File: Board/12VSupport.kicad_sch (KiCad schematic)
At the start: 33 parts, among them J1 12V, J2 BATT, J3 BUCK_IN, J4 BUCK_OUT, J5 BOOST_IN, J6 BOOST_OUT, J8 HEATER, K1 SLA-05VDC-SL-C, K2 SLA-05VDC-SL-C, K3 SLA-05VDC-SL-C, K4 SLA-05VDC-SL-C, Q1 BSS138, Q2 BSS138, Q3 MMBF170, Q4 IRLR7843, U1 LM2596S-5, U4 ACS712xLCTR-20A

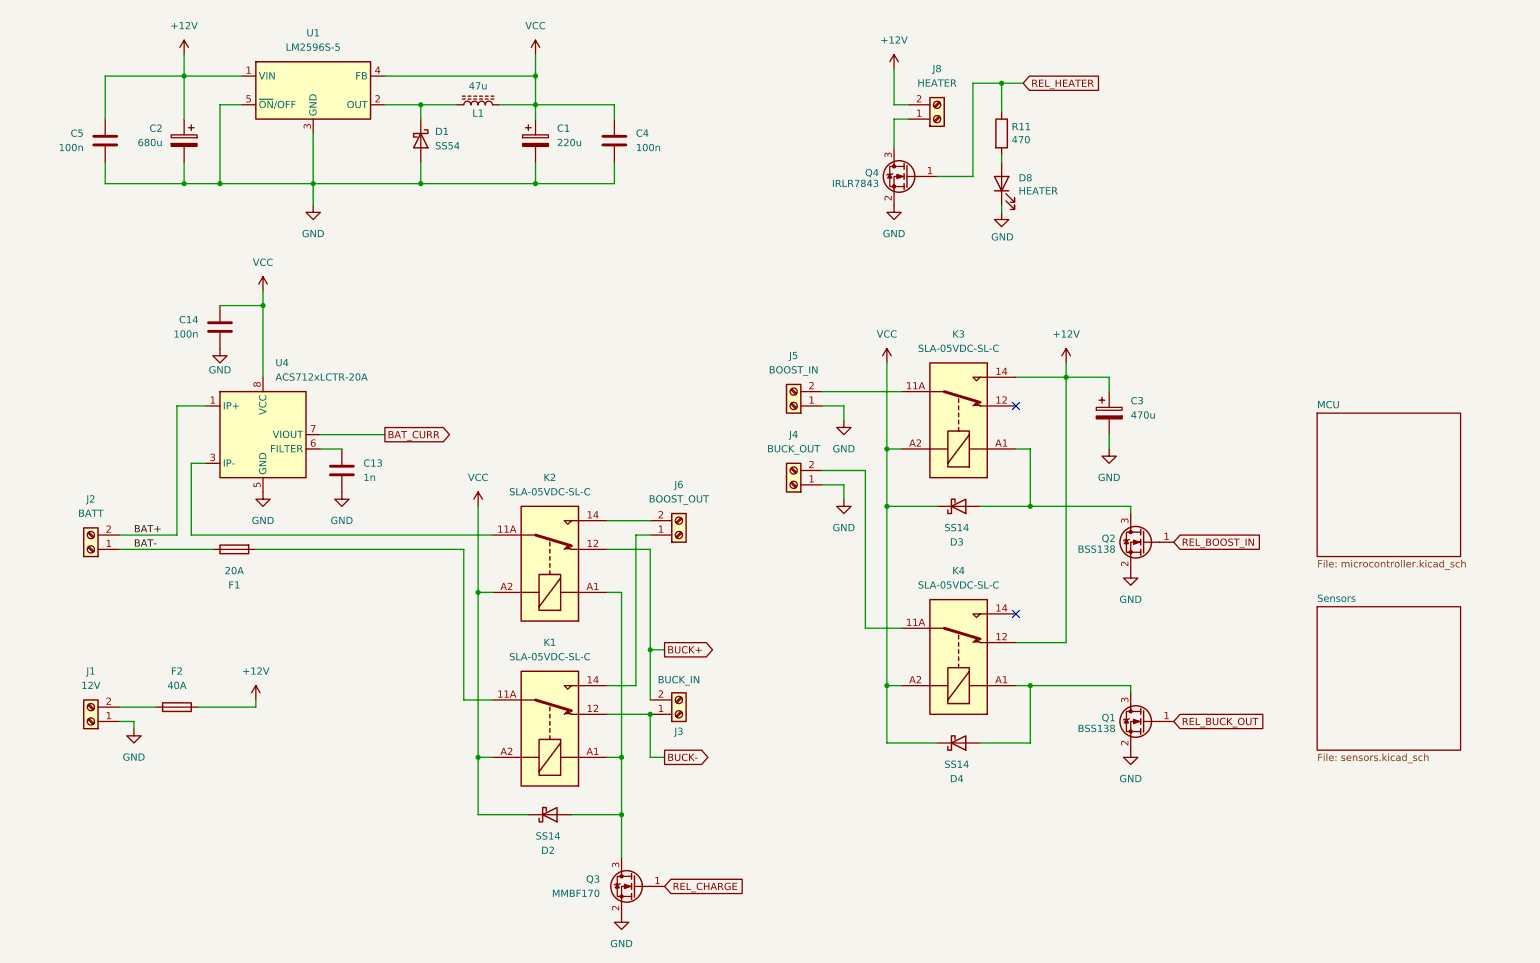
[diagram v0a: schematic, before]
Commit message: WIP
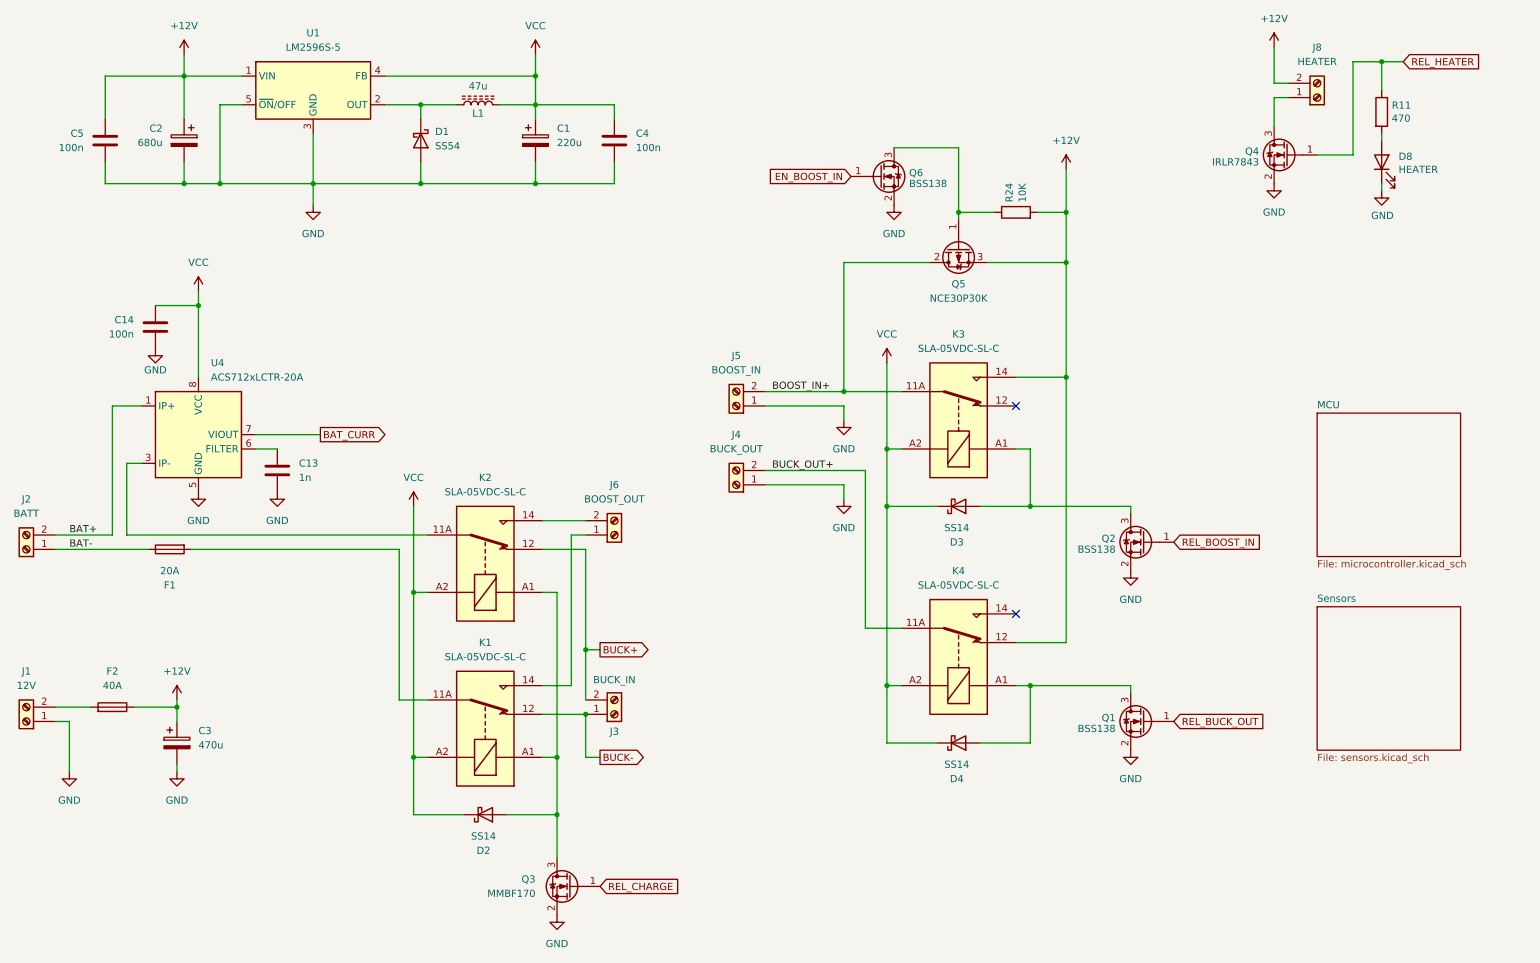
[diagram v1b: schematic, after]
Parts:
- added Q5: NCE30P30K, Package_TO_SOT_SMD:TO-252-2, symbol Transistor_FET:QM6015D
- added Q6: BSS138, Package_TO_SOT_SMD:SOT-23, symbol Transistor_FET:BSS138
- added R24: 10K, Resistor_SMD:R_0805_2012Metric, symbol Device:R
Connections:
- net +12V: now also Q5.3 (S), R24.2
- net GND: now also Q6.2 (S)
- net BUCK_OUT+: now reaches J4.2 (Pin_2), K4.11A, K4.11B
- net BOOST_IN+: now reaches J5.2 (Pin_2), K3.11A, K3.11B
- net BOOST_IN+: now also Q5.2 (D)
- new net: Q5.1 (G), Q6.3 (D), R24.1
- new net EN_BOOST_IN: Q6.1 (G)
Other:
- moved on the sheet: C13, C14, C3, D2, D8, F1, F2, J1, J2, J3, J4, J5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
